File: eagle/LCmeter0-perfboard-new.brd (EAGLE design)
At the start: 63.5 x 48.3 mm, 25 parts, among them IC1 PIC16F876A-X/SP, K2 DS2Y, Q1 20MHz, Q2 BC548, SW1 SPST, SW2 DPDT

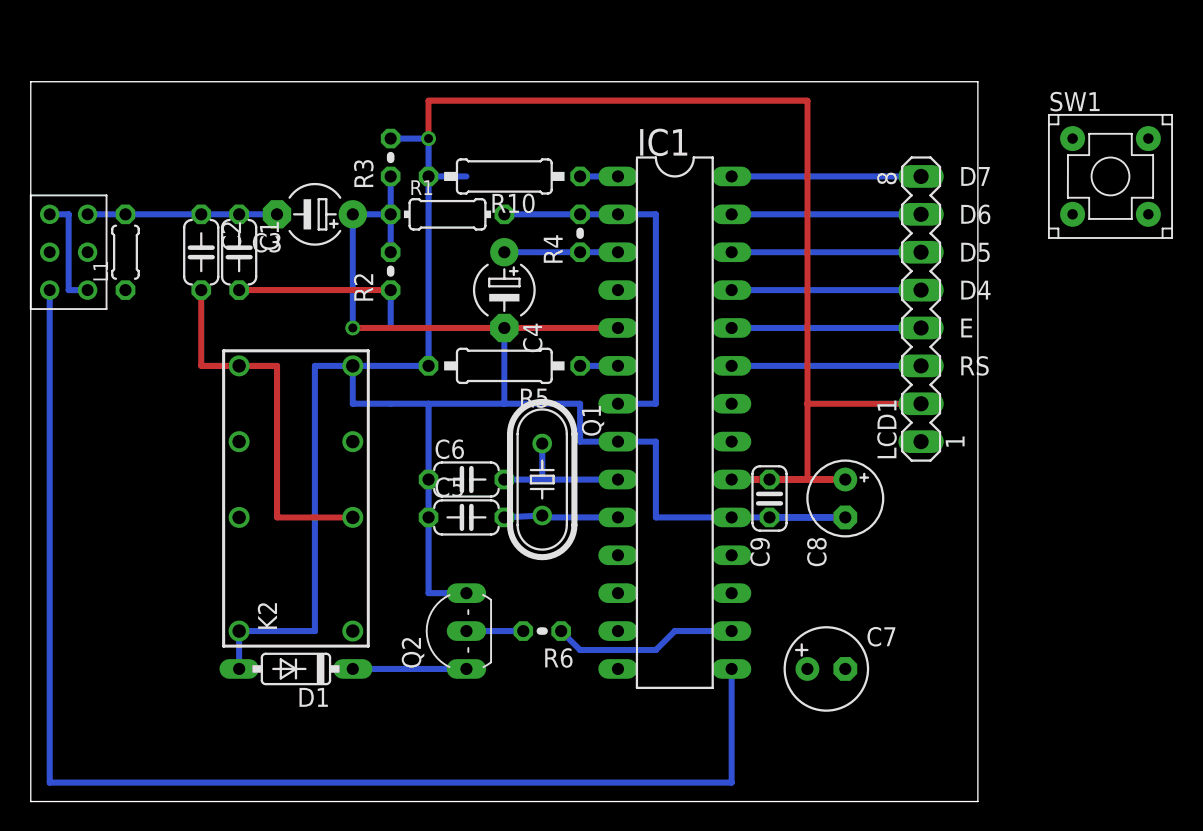
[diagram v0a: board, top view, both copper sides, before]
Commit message: ...
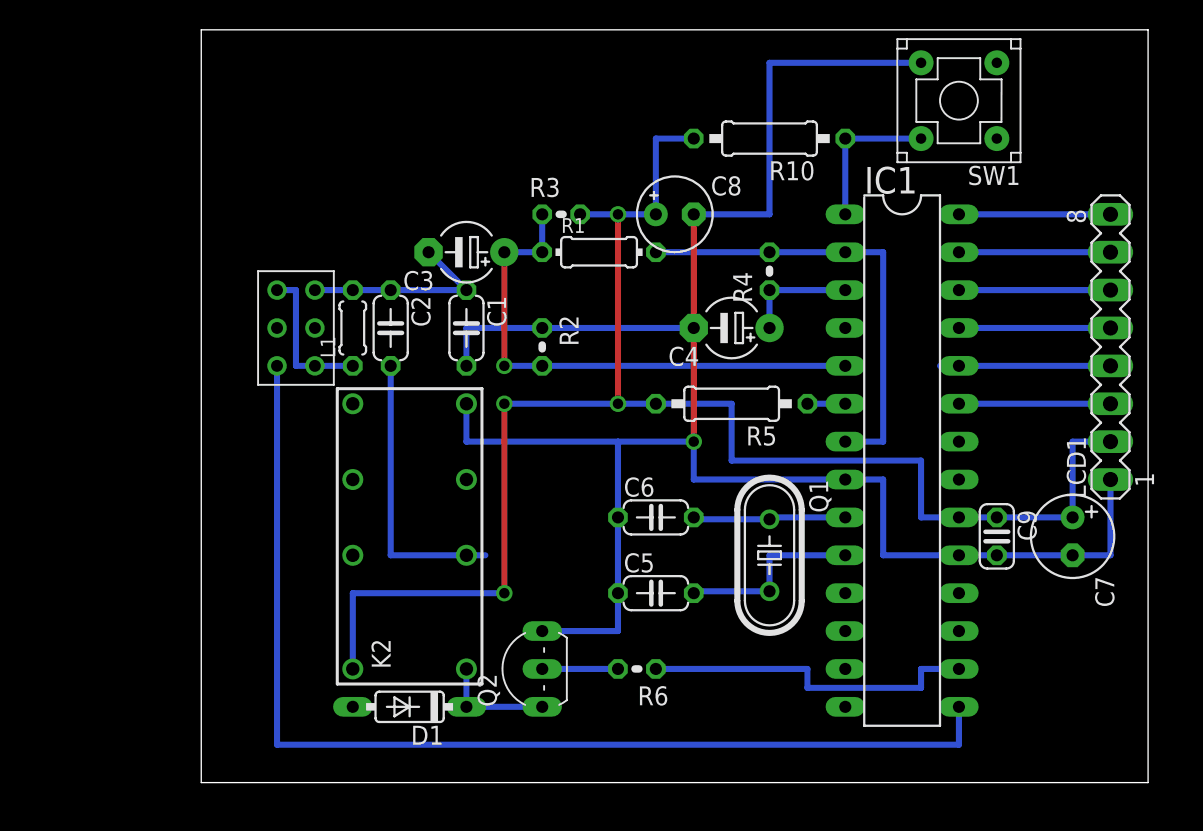
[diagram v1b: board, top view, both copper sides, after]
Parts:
- moved C8 22.2 mm to (31.8, 38.1), turned to 0 degrees
- moved C7 18.8 mm to (58.4, 16.5), turned to 270 degrees
- moved R10 18.0 mm to (38.1, 43.2)
- moved C1 16.1 mm to (17.8, 30.5)
- moved L1 16.1 mm to (10.2, 30.5)
- moved Q1 16.1 mm to (38.1, 15.2)
- moved SW2 16.1 mm to (6.35, 30.5)
- moved C4 15.5 mm to (35.6, 30.5), turned to 180 degrees
- moved R5 15.5 mm to (35.6, 25.4)
- moved C9 15.5 mm to (53.3, 16.5)
- moved IC1 15.5 mm to (47.0, 21.6)
- moved C2 13.7 mm to (12.7, 30.5)
- moved C5 13.7 mm to (30.5, 12.7)
- moved LCD1 13.0 mm to (61.0, 29.2)
- moved R4 13.0 mm to (38.1, 34.3)
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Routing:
- net GND: track 88.9 -> 134.6 mm, vias 0 -> 1
- net VCC: track 132.1 -> 106.7 mm, vias 1 -> 4
- net /LC: track 86.4 -> 73.7 mm
- net RC5: track 12.5 -> 22.9 mm
- net /MCLR: track 2.54 -> 10.2 mm
- net C2_CON: track 25.4 -> 19.1 mm
- net A0: track 25.4 -> 30.5 mm
- net OSC2: track 7.75 -> 12.7 mm
- net N$7: track 7.62 -> 10.2 mm
- net A3: track 33.0 -> 35.6 mm
- net RS: track 12.7 -> 10.2 mm
- net D7: track 12.7 -> 10.2 mm
- net D6: track 12.7 -> 10.2 mm
- net D5: track 12.7 -> 10.2 mm
- net D4: track 12.7 -> 10.2 mm
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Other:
- board size 63.5 x 48.3 mm -> 63.5 x 50.5 mm
- board text removed: "D4"
- board text removed: "D5"
- board text removed: "D6"
- board text removed: "D7"
- board text removed: "E"
- board text removed: "RS"
